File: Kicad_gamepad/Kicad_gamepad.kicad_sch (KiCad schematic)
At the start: 28 parts, among them J1 USB_A, SW1 SW_Push, SW10 SW_Push, SW11 SW_Push, SW2 SW_Push, SW3 SW_Push, SW4 SW_Push, SW5 SW_Push, SW6 SW_Push, SW7 SW_Push, SW8 SW_Push, SW9 SW_Push, U1 PIC18F4550-IPT, Y1 Crystal

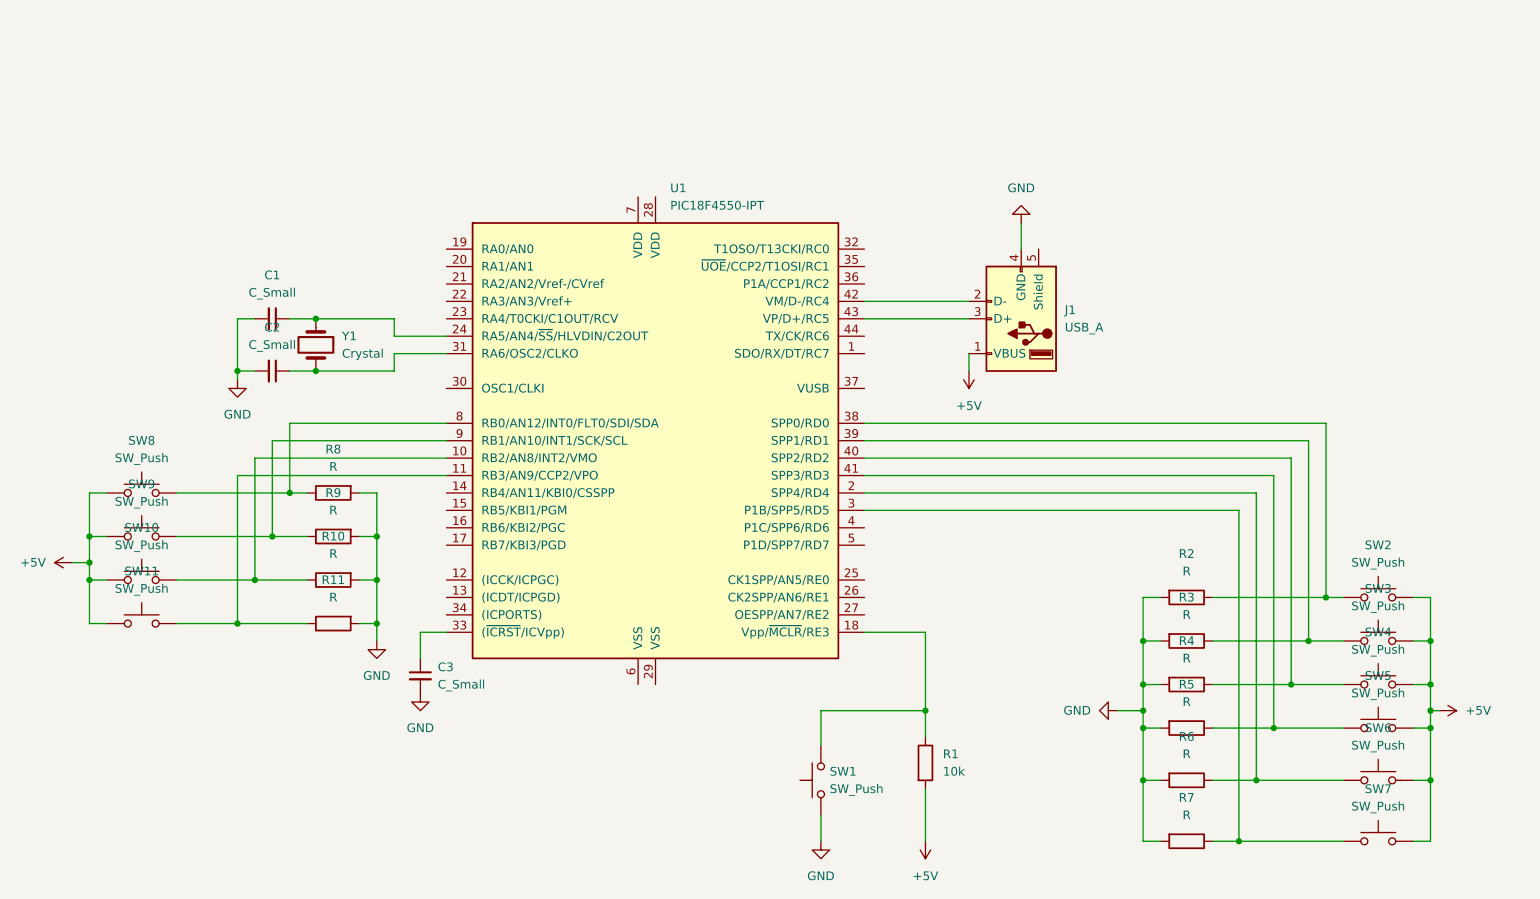
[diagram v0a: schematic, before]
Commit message: Kicad prueba 1
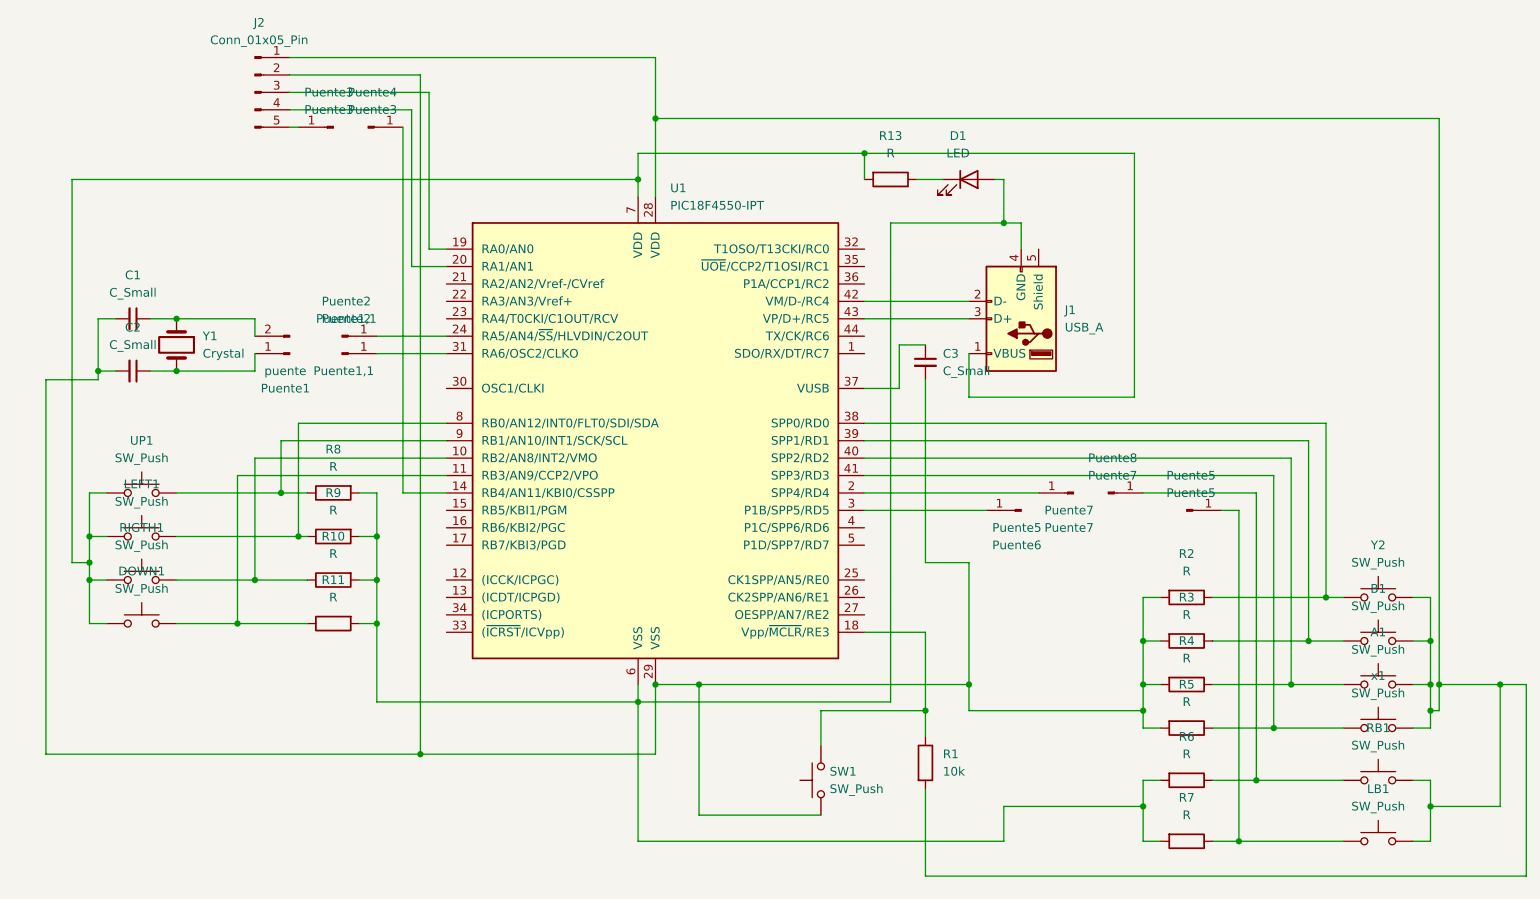
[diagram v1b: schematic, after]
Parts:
- added D1: LED, LED_THT:LED_D3.0mm, symbol Device:LED
- added J2: Conn_01x05_Pin, Connector_JST:JST_VH_B5P-VH_1x05_P3.96mm_Vertical, symbol Connector:Conn_01x05_Pin
- added Puente1: puente, Connector_PinHeader_2.54mm:PinHeader_1x02_P2.54mm_Vertical, symbol Connector:Conn_01x02_Pin
- added Puente1,1: Puente1,1, Connector_PinHeader_2.54mm:PinHeader_1x01_P2.54mm_Vertical, symbol Connector:Conn_01x01_Pin
- added Puente2: Puente2, Connector_PinHeader_2.54mm:PinHeader_1x01_P2.54mm_Vertical, symbol Connector:Conn_01x01_Pin
- added Puente3, Puente4: Puente3, Connector_PinHeader_2.54mm:PinHeader_1x01_P2.54mm_Vertical, symbol Connector:Conn_01x01_Pin
- added Puente5, Puente6: Puente5, Connector_PinHeader_2.54mm:PinHeader_1x01_P2.54mm_Vertical, symbol Connector:Conn_01x01_Pin
- added Puente7, Puente8: Puente7, Connector_PinHeader_2.54mm:PinHeader_1x01_P2.54mm_Vertical, symbol Connector:Conn_01x01_Pin
- added R13: R, Resistor_THT:R_Axial_DIN0207_L6.3mm_D2.5mm_P10.16mm_Horizontal, symbol Device:R
- A1: renamed from SW4; footprint (none) -> Button_Switch_THT:SW_PUSH_6mm
- B1: renamed from SW3; footprint (none) -> Button_Switch_THT:SW_PUSH_6mm
- C1, C2: footprint (none) -> Capacitor_THT:C_Disc_D6.0mm_W2.5mm_P5.00mm
- C3: footprint (none) -> Capacitor_THT:C_Disc_D5.0mm_W2.5mm_P2.50mm
- DOWN1: renamed from SW11; footprint (none) -> Button_Switch_THT:SW_PUSH_6mm
- LB1: renamed from SW7; footprint (none) -> Button_Switch_THT:SW_PUSH_6mm
- LEFT1: renamed from SW9; footprint (none) -> Button_Switch_THT:SW_PUSH_6mm
- R1, R2, R3, R4, R5, R6, R7: footprint (none) -> Resistor_THT:R_Axial_DIN0207_L6.3mm_D2.5mm_P10.16mm_Horizontal
- R10, R11, R8, R9: footprint (none) -> Resistor_THT:R_Axial_DIN0204_L3.6mm_D1.6mm_P7.62mm_Horizontal
- RB1: renamed from SW6; footprint (none) -> Button_Switch_THT:SW_PUSH_6mm
- RIGTH1: renamed from SW10; footprint (none) -> Button_Switch_THT:SW_PUSH_6mm
- SW1: footprint (none) -> Button_Switch_THT:SW_PUSH_6mm
- UP1: renamed from SW8; footprint (none) -> Button_Switch_THT:SW_PUSH_6mm
- Y1: footprint (none) -> Crystal:Crystal_HC52-U_Vertical
- Y2: renamed from SW2; footprint (none) -> Button_Switch_THT:SW_PUSH_6mm
- x1: renamed from SW5; footprint (none) -> Button_Switch_THT:SW_PUSH_6mm
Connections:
- net at LB1.1, R7.1: now also Puente5.1 (Pin_1); no longer U1.3 (P1B/SPP5/RD5)
- net at R8.1, UP1.1: now also U1.9 (RB1/AN10/INT1/SCK/SCL); no longer U1.8 (RB0/AN12/INT0/FLT0/SDI/SDA)
- net at C1.1, Y1.1: now also Puente1.2 (Pin_2); no longer U1.24 (RA5/AN4/~{SS}/HLVDIN/C2OUT)
- net at C2.1, Y1.2: now also Puente1.1 (Pin_1); no longer U1.31 (RA6/OSC2/CLKO)
- net at LEFT1.1, R9.1: now also U1.8 (RB0/AN12/INT0/FLT0/SDI/SDA); no longer U1.9 (RB1/AN10/INT1/SCK/SCL)
- net at C3.1: now also U1.37 (VUSB); no longer U1.33 ((~{ICRST}/ICVpp))
- net at R6.1, RB1.1: now also Puente8.1 (Pin_1); no longer U1.2 (SPP4/RD4)
- net at U1.14 (RB4/AN11/KBI0/CSSPP): now also Puente4.1 (Pin_1)
- net at U1.19 (RA0/AN0): now also J2.3 (Pin_3)
- net at U1.20 (RA1/AN1): now also J2.4 (Pin_4)
- net at U1.28 (VDD): now also A1.2, B1.2, LB1.2, R1.2, RB1.2, Y2.2, x1.2, J2.1 (Pin_1)
- net at U1.29 (VSS): now also C1.2, C2.2, C3.2, R2.2, R3.2, R4.2, R5.2, SW1.1, J2.2 (Pin_2)
- net at U1.6 (VSS): now also J1.4 (GND), R10.2, R11.2, R6.2, R7.2, R8.2, R9.2, D1.2 (A)
- net at U1.7 (VDD): now also DOWN1.2, J1.1 (VBUS), LEFT1.2, RIGTH1.2, UP1.2, R13.2
- removed net +5V: A1.2, B1.2, DOWN1.2, J1.1 (VBUS), LB1.2, LEFT1.2, R1.2, RB1.2, RIGTH1.2, UP1.2, Y2.2, x1.2
- removed net GND: C1.2, C2.2, C3.2, J1.4 (GND), R10.2, R11.2, R2.2, R3.2, R4.2, R5.2, R6.2, R7.2, R8.2, R9.2, SW1.1
- new net: Puente7.1 (Pin_1), U1.2 (SPP4/RD4)
- new net: Puente2.1 (Pin_1), U1.24 (RA5/AN4/~{SS}/HLVDIN/C2OUT)
- new net: Puente1,1.1 (Pin_1), U1.31 (RA6/OSC2/CLKO)
- new net: D1.1 (K), R13.1
- new net: Puente6.1 (Pin_1), U1.3 (P1B/SPP5/RD5)
- new net: J2.5 (Pin_5), Puente3.1 (Pin_1)
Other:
- moved on the sheet: C1, C2, C3, Y1
